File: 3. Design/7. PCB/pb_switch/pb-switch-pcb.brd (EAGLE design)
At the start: 16 x 13.8 mm, 9 parts, among them SW1 B3F-1000

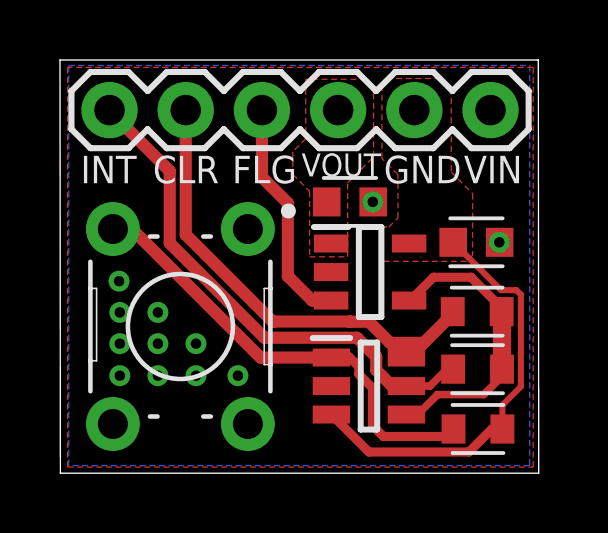
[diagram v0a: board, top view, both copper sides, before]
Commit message: ADD|UPDT: Exported new and corrected old 3D models, 2D models and technical drawings of all  PCBs
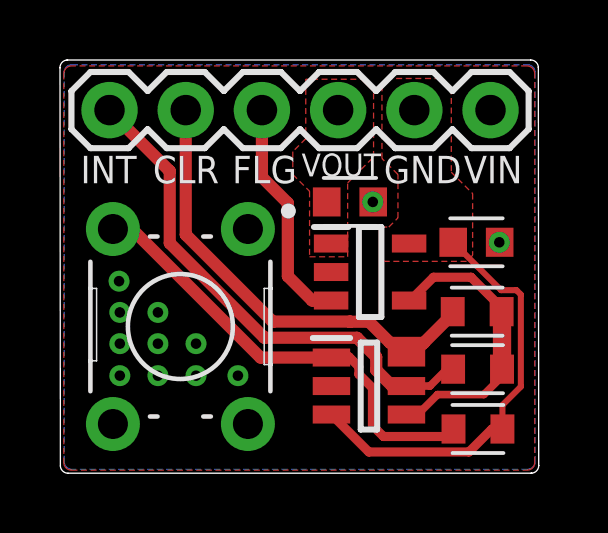
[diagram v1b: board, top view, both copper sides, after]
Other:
- outline, holes or cut-outs redrawn
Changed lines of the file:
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@@
 </layers>
 <board>
-<fusionsync huburn="a.YnVzaW5lc3M6YWx1bm9zNjU4" projecturn="a.YnVzaW5lc3M6YWx1bm9zNjU4I0QyMDIwMTEyNjM1NzA0MDM1MQ" f3durn="urn:adsk.wipprod:dm.lineage:3VlmRX1nQs2zZRRoKQ1P4A" pcbguid="" lastpulledtime="" lastsyncedchangeguid="" latestrevisionid="f04446ce-984e-4f57-afe4-5e06ea0c3ac4" lastsyncedrevisionid="f04446ce-984e-4f57-afe4-5e06ea0c3ac4" lastboardhashguid="f9ee74f5-27dd-6472-24e2-1c3aec2db798" lastpushedtime="2020-12-18T12:14:57Z" linktopcb3d="true"/>
+<fusionsync huburn="a.YnVzaW5lc3M6YWx1bm9zNjU4" projecturn="a.YnVzaW5lc3M6YWx1bm9zNjU4I0QyMDIwMTEyNjM1NzA0MDM1MQ" f3durn="urn:adsk.wipprod:dm.lineage:3VlmRX1nQs2zZRRoKQ1P4A" pcbguid="" lastpulledtime="2020-12-21T00:10:31Z" lastsyncedchangeguid="" latestrevisionid="395f5c64-1056-4925-aef1-c0004189c743" lastsyncedrevisionid="bd750037-602d-4ef0-af0e-b9f6cfe8811f" lastboardhashguid="253df748-d07a-61a5-b856-ef57312ef0c4" lastpushedtime="2020-12-20T23:26:12Z" linktopcb3d="true"/>
 <plain>
-<wire x1="0" y1="0" x2="15.9446" y2="0" width="0" layer="20"/>
-<wire x1="15.9446" y1="0" x2="15.9319" y2="13.7731" width="0" layer="20"/>
-<wire x1="15.9319" y1="13.7731" x2="-0.0127" y2="13.7731" width="0" layer="20"/>
-<wire x1="-0.0127" y1="13.7731" x2="0" y2="0" width="0" layer="20"/>
 <text x="10.7823" y="9.6647" size="0.9144" layer="21" font="vector" ratio="18">GND</text>
 <text x="13.4493" y="9.6647" size="0.9144" layer="21" font="vector" ratio="18">VIN</text>
@@
 <text x="3.0861" y="9.6647" size="0.9144" layer="21" font="vector" ratio="18">CLR</text>
 <text x="0.6731" y="9.6647" size="0.9144" layer="21" font="vector" ratio="18">INT</text>
+<wire x1="0.2538" y1="0" x2="15.6904" y2="0" width="0" layer="20"/>
+<wire x1="15.6904" y1="0" x2="15.7125" y2="0.001" width="0" layer="20"/>
+<wire x1="15.7125" y1="0.001" x2="15.9444" y2="0.254" width="0" layer="20" curve="85.0001"/>
+<wire x1="15.9444" y1="0.254" x2="15.9444" y2="0.2542" width="0" layer="20"/>
+<wire x1="15.9444" y1="0.2542" x2="15.9321" y2="13.5189" width="0" layer="20"/>
+<wire x1="15.9321" y1="13.5189" x2="15.9312" y2="13.5411" width="0" layer="20"/>
+<wire x1="15.9312" y1="13.5411" x2="15.6781" y2="13.7731" width="0" layer="20" curve="84.9471"/>
+<wire x1="15.6781" y1="13.7731" x2="0.2415" y2="13.7731" width="0" layer="20"/>
+<wire x1="0.2415" y1="13.7731" x2="0.2194" y2="13.7721" width="0" layer="20"/>
+<wire x1="0.2194" y1="13.7721" x2="-0.0125" y2="13.5191" width="0" layer="20" curve="85.0001"/>
+<wire x1="-0.0125" y1="13.5191" x2="-0.0125" y2="13.5189" width="0" layer="20"/>
+<wire x1="-0.0125" y1="13.5189" x2="-0.0002" y2="0.2542" width="0" layer="20"/>
+<wire x1="-0.0002" y1="0.2542" x2="0.0007" y2="0.232" width="0" layer="20"/>
+<wire x1="0.0007" y1="0.232" x2="0.2538" y2="0" width="0" layer="20" curve="84.9471"/>
 </plain>
 <attributes>
@@
 <attribute name="VALUE" x="0.3683" y="10.0711" size="0.6096" layer="27" font="vector" ratio="20"/>
 </element>
-<element name="C2" library="Capacitor" library_urn="urn:adsk.eagle:library:16290819" package="CAPC1608X85" package3d_urn="urn:adsk.eagle:package:16290898/2" value="100n [0603]" x="13.8684" y="7.6962" smashed="yes">
+<element name="C2" library="Capacitor" library_urn="urn:adsk.eagle:library:16290819" package="CAPC1608X85" package3d_urn="urn:adsk.eagle:package:16290898/2" override_package3d_urn="urn:adsk.eagle:package:25496701/2" override_package_urn="urn:adsk.eagle:footprint:16290847/2" value="100n [0603]" x="13.8684" y="7.6962" smashed="yes">
 <attribute name="CATEGORY" value="Capacitor" x="11.8618" y="7.6962" size="1.778" layer="27" display="off"/>
 <attribute name="MANUFACTURER" value="" x="11.8618" y="7.6962" size="1.778" layer="27" display="off"/>
@@
 <attribute name="VOLTAGE_RATING" value="" x="11.8618" y="7.6962" size="1.778" layer="27" display="off"/>
 </element>
-<element name="C1" library="Capacitor" library_urn="urn:adsk.eagle:library:16290819" package="CAPC1608X85" package3d_urn="urn:adsk.eagle:package:16290898/2" value="100n [0603]" x="9.652" y="9.0424" smashed="yes">
+<element name="C1" library="Capacitor" library_urn="urn:adsk.eagle:library:16290819" package="CAPC1608X85" package3d_urn="urn:adsk.eagle:package:16290898/2" override_package3d_urn="urn:adsk.eagle:package:25496704/2" override_package_urn="urn:adsk.eagle:footprint:16290847/2" value="100n [0603]" x="9.652" y="9.0424" smashed="yes">
 <attribute name="CATEGORY" value="Capacitor" x="8.3058" y="9.0424" size="1.778" layer="27" display="off"/>
 <attribute name="MANUFACTURER" value="" x="8.3058" y="9.0424" size="1.778" layer="27" display="off"/>
@@
 <contactref element="PB_CTRL" pad="2"/>
 <polygon width="0.127" layer="1" thermals="no" rank="2">
-<vertex x="0.2413" y="13.5255"/>
-<vertex x="0.2413" y="0.2032"/>
-<vertex x="15.7607" y="0.2032"/>
-<vertex x="15.7607" y="13.5255"/>
+<vertex x="0.1143" y="13.3223"/>
+<vertex x="0.1143" y="0.3556" curve="90"/>
+<vertex x="0.3683" y="0.1016"/>
+<vertex x="15.5575" y="0.1016" curve="90"/>
+<vertex x="15.8115" y="0.3556"/>
+<vertex x="15.8115" y="13.3223" curve="90"/>
+<vertex x="15.5575" y="13.5763"/>
+<vertex x="0.3683" y="13.5763" curve="90"/>
 </polygon>
 <contactref element="SW1" pad="1"/>
@@
 <contactref element="J2" pad="6"/>
 <polygon width="0.1524" layer="16" thermals="no">
-<vertex x="0.2794" y="13.589"/>
-<vertex x="15.6464" y="13.589"/>
-<vertex x="15.6464" y="0.254"/>
-<vertex x="0.2794" y="0.254"/>
+<vertex x="15.5702" y="0.127"/>
+<vertex x="0.381" y="0.127" curve="-90"/>
+<vertex x="0.127" y="0.381"/>
+<vertex x="0.127" y="13.3604" curve="-90"/>
+<vertex x="0.381" y="13.6144"/>
+<vertex x="15.5702" y="13.6144" curve="-90"/>
+<vertex x="15.8242" y="13.3604"/>
+<vertex x="15.8242" y="0.381" curve="-90"/>
 </polygon>
 <via x="1.9812" y="5.3594" extent="1-16" drill="0.35" diameter="0.7"/>
@@
 <contactref element="R6" pad="2"/>
 <contactref element="PB_CTRL" pad="4"/>
-<contactref element="PS1" pad="4"/>
 <wire x1="14.7217" y1="3.4671" x2="14.7217" y2="3.2258" width="0.254" layer="1"/>
 <wire x1="14.7217" y1="3.2258" x2="14.11645" y2="2.62055" width="0.254" layer="1"/>
@@
 <wire x1="11.9082875" y1="1.9548" x2="11.5353" y2="1.9548" width="0.254" layer="1"/>
 <wire x1="12.5740375" y1="2.62055" x2="11.9082875" y2="1.9548" width="0.254" layer="1"/>
-<wire x1="11.65996875" y1="5.7556" x2="11.6251" y2="5.7556" width="0.3048" layer="1"/>
-<wire x1="12.43651875" y1="6.53215" x2="11.65996875" y2="5.7556" width="0.3048" layer="1"/>
+<wire x1="11.65996875" y1="5.7556" x2="12.43651875" y2="6.53215" width="0.3048" layer="1"/>
 <wire x1="12.43651875" y1="6.53215" x2="13.68865" y2="6.53215" width="0.3048" layer="1"/>
 <wire x1="13.68865" y1="6.53215" x2="14.7217" y2="5.4991" width="0.3048" layer="1"/>
@@
 <wire x1="14.709" y1="5.3848" x2="14.7217" y2="5.3721" width="0.6096" layer="1"/>
 <wire x1="14.7217" y1="5.3721" x2="14.7217" y2="3.4671" width="0.6096" layer="1"/>
+<contactref element="PS1" pad="4"/>
+<wire x1="11.6251" y1="5.7556" x2="11.65996875" y2="5.7556" width="0.1524" layer="1"/>
 </signal>
 <signal name="VIN">
